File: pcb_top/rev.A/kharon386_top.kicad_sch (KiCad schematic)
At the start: 153 parts, among them J1 PJ-322, J2 Vol. Btns, J3 Conn_02x07_Odd_Even, J4 ESP, J5 PC104_16, J6 PC104, SW1 VGA Config, U1 1117-5.0, U11 MT4C4256, U12 MT4C4256, U13 MT4C4256, U14 MT4C4256, U2 NE5532DR, U3 74HCT138, U4 ES1868F, U5 TVGA9000I, U6 SAM2695, U7 27C256, U8 1117-5.0, U9 1117-3.3, Y1 40 MHz, Y2 12 MHz

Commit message: wip pcb rev.A
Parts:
- C39, C40, C42, C45, C49: symbol Device:CP -> Device:C_Polarized
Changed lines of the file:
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@@
     (pin "2")
   )
-  (symbol (lib_id "Device:CP") (at 466.725 250.19 0) (unit 1)
+  (symbol (lib_id "Device:C_Polarized") (at 466.725 250.19 0) (unit 1)
     (in_bom yes) (on_board yes)
     (property "Reference" "C42" (id 0) (at 468.63 248.285 0)
@@
     (pin "1")
   )
-  (symbol (lib_id "Device:CP") (at 440.055 232.41 0) (unit 1)
+  (symbol (lib_id "Device:C_Polarized") (at 440.055 232.41 0) (unit 1)
     (in_bom yes) (on_board yes)
     (property "Reference" "C40" (id 0) (at 441.96 230.505 0)
@@
     (pin "1")
   )
-  (symbol (lib_id "Device:CP") (at 466.725 269.875 0) (unit 1)
+  (symbol (lib_id "Device:C_Polarized") (at 466.725 269.875 0) (unit 1)
     (in_bom yes) (on_board yes)
     (property "Reference" "C49" (id 0) (at 468.63 267.97 0)
@@
     (pin "1")
   )
-  (symbol (lib_id "Device:CP") (at 442.595 313.055 0) (unit 1)
+  (symbol (lib_id "Device:C_Polarized") (at 442.595 313.055 0) (unit 1)
     (in_bom yes) (on_board yes)
     (property "Reference" "C45" (id 0) (at 444.5 311.15 0)
@@
     (pin "9")
   )
-  (symbol (lib_id "Device:CP") (at 466.725 232.41 0) (unit 1)
+  (symbol (lib_id "Device:C_Polarized") (at 466.725 232.41 0) (unit 1)
     (in_bom yes) (on_board yes)
     (property "Reference" "C39" (id 0) (at 468.63 230.505 0)

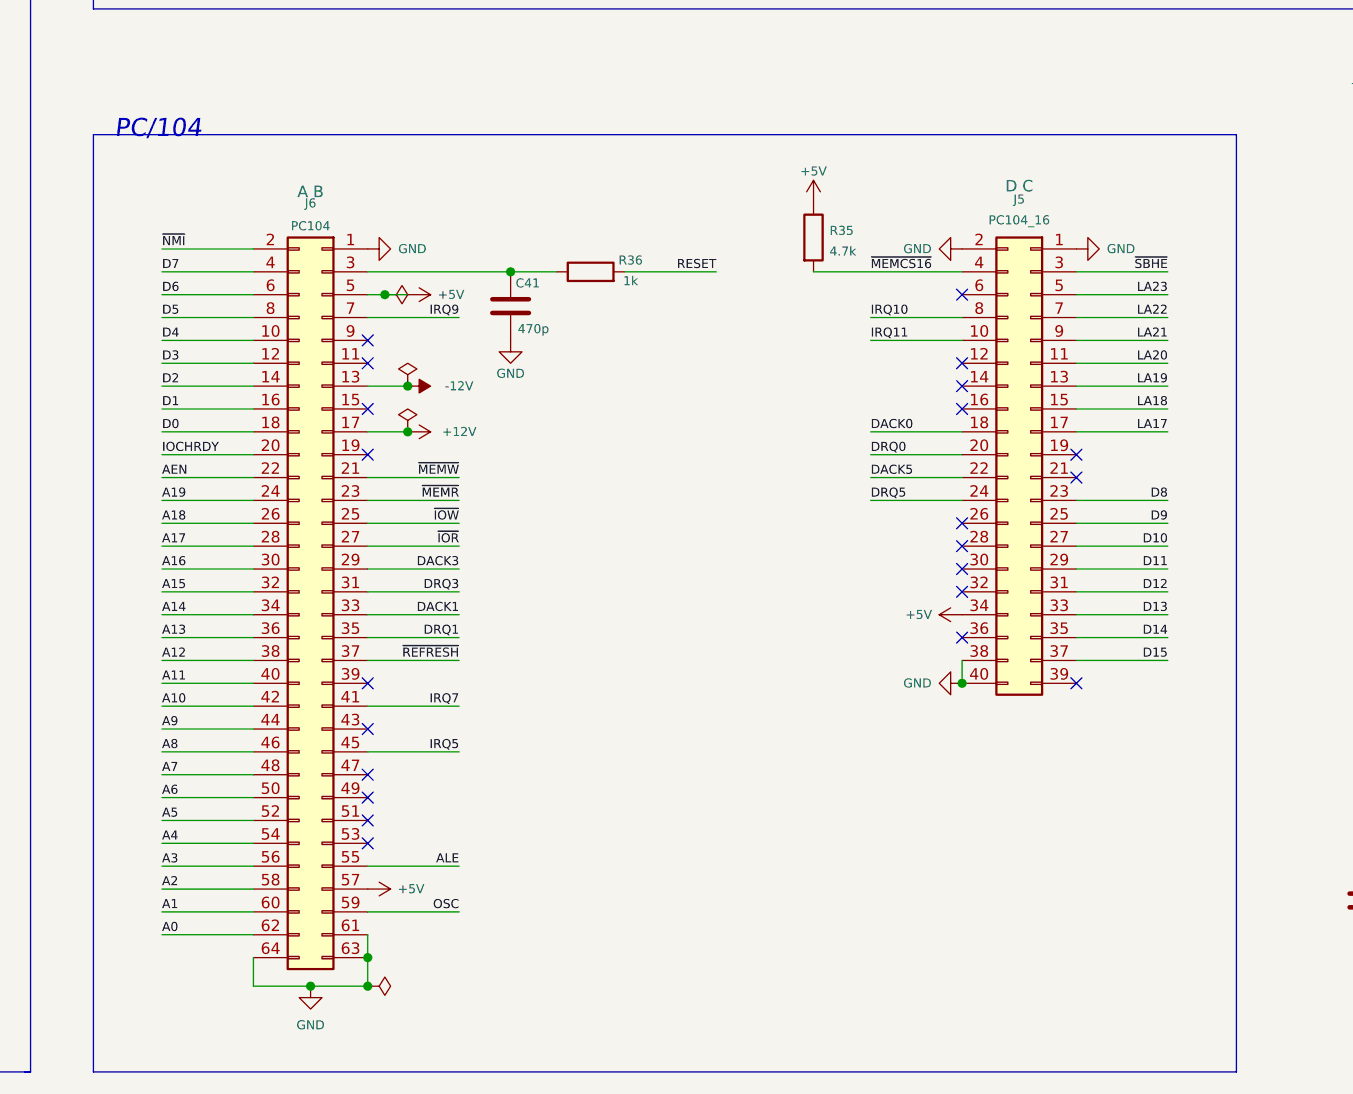
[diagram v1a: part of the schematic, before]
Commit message: wip pcb rev.A
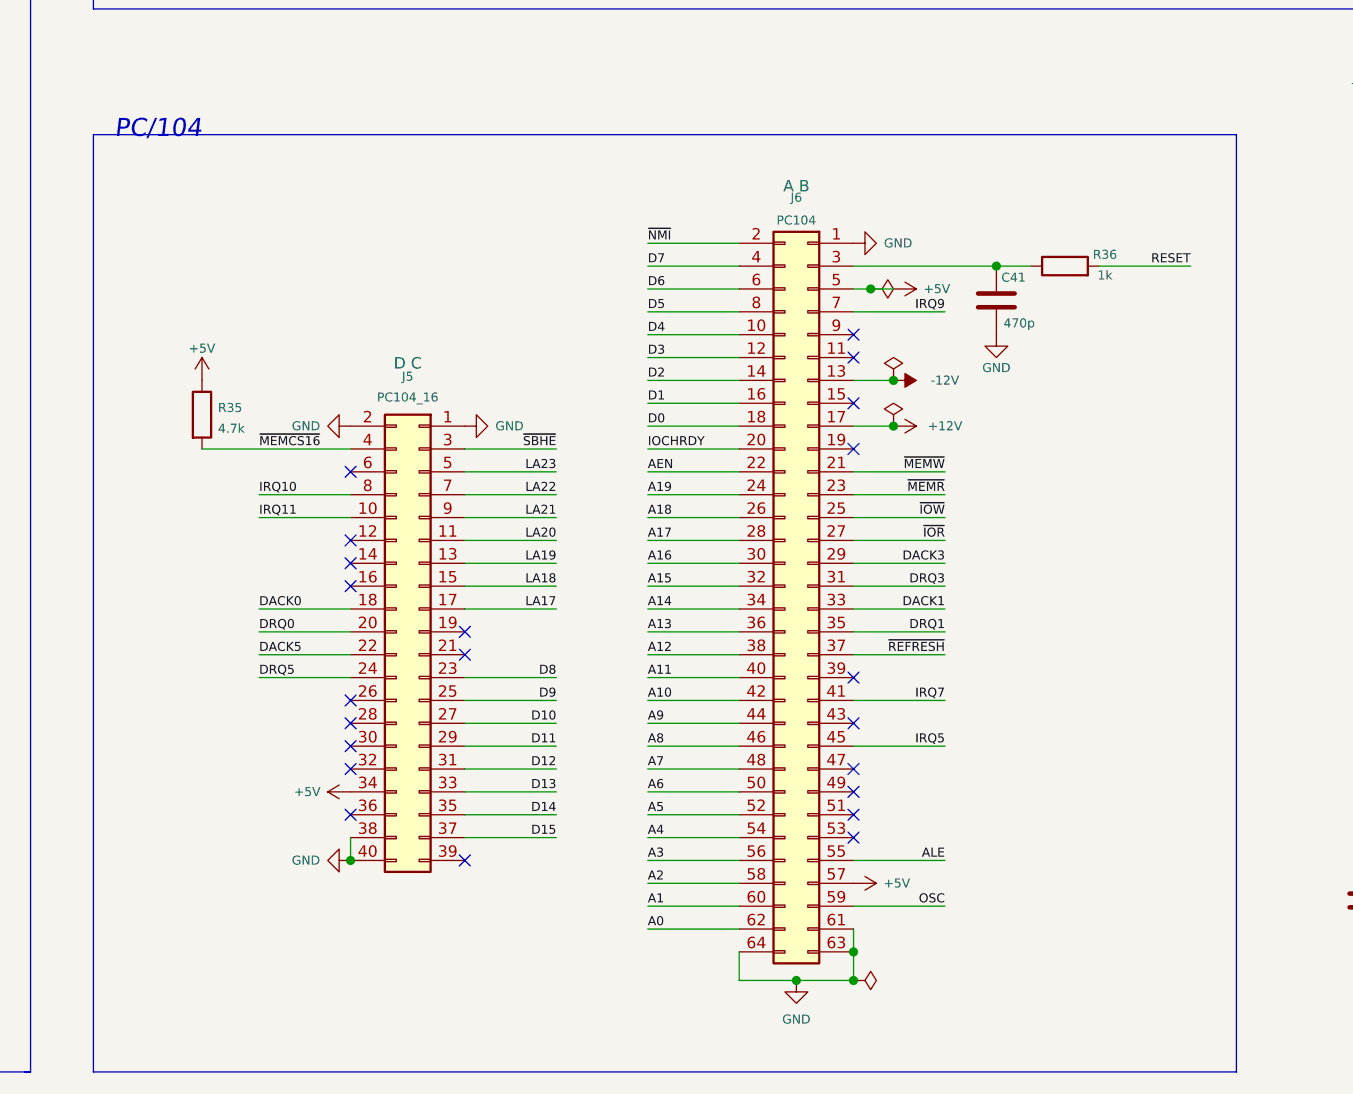
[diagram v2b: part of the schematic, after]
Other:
- moved on the sheet: C41, J5, J6, R35, R36
